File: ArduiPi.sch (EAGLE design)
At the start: 59 parts, among them IC1 DS2482-100S, IC2 AVR-MEGA8-PPTH, J1 VIN, J3 ISP, Q1 BS170, Q2 BS170, Q3 BS170, Q4 BS170, U1 LD1117 3V3, U2 78M05, U3 TXB0108, U4 TXB0108, Y1 16MHz

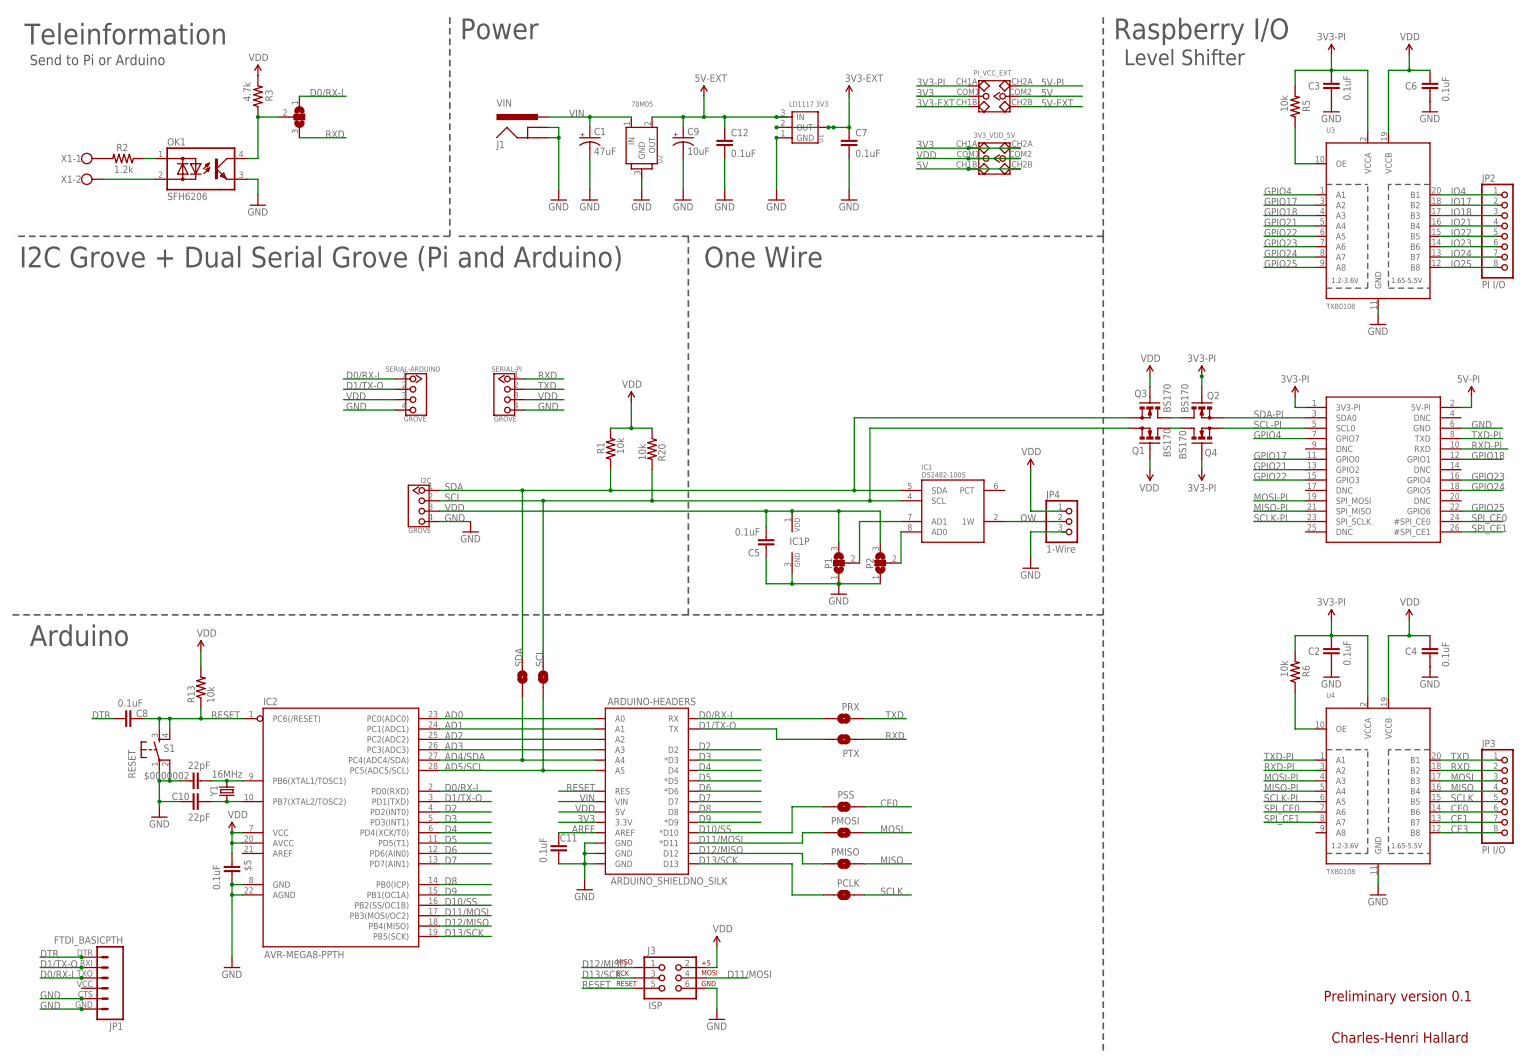
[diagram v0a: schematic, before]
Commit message: Final Design
Final Design
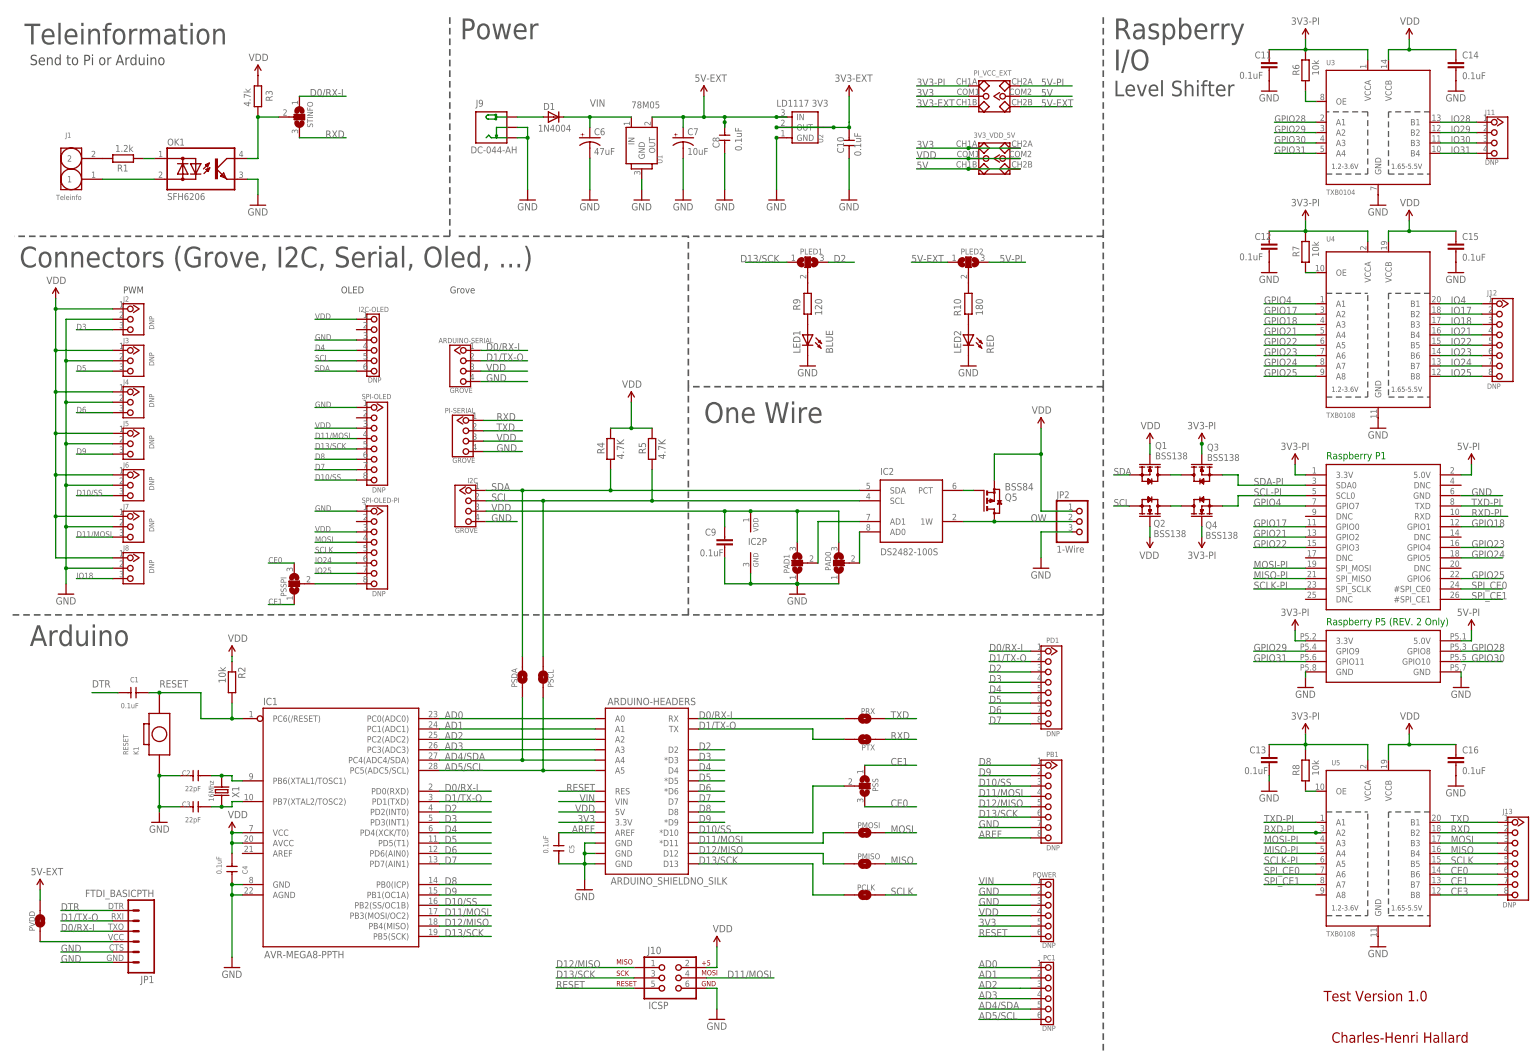
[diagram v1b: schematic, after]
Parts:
- removed $0000002: 22pF, SparkFun:CAPPTH2
- removed $5: 0.1uF, SparkFun:CAPPTH2
- removed JP3: PI I/O, adafruit:PINHD-1X8BIG
- removed JP4: 1-Wire, adafruit:PINHD-1X3
- removed P1, P2: (no value), Seeedstudio-Discreter.rpt:PAD-SOLDERJUMPER-2WAYT
- removed R13, R20: 10k, SparkFun:RESISTORAXIAL-0.3
- removed RASPBERRY: RASPBERRYPI_BB, microbuilder:RASPBERRYPI_BB
- removed S1: RESET, SparkFun:TAC_SWITCHPTH
- removed SERIAL-ARDUINO, SERIAL-PI: GROVE, Connector:TWIG-2.0-LEADED
- removed Y1: 16MHz, SparkFun:CRYSTALHC49US
- added ARDUINO-SERIAL, PI-SERIAL: GROVE, Connector:TWIG-2.0-LEADED
- added C13, C14, C15, C16: 0.1uF, resistor:C-EUC0603
- added D1: 1N4004, adafruit:1N4004
- added I2C-OLED, PC1, POWER: DNP, Seeedstudio-Connector:HEADER-6P-2.54
- added J10: ICSP, SparkFun:AVR_SPI_PRG_6PTH
- added J11: DNP, Seeedstudio-Connector:HEADER-4P-80/40MIL
- added J12, J13, PB1, PD1, SPI-OLED, SPI-OLED-PI: DNP, Seeedstudio-Connector:HEADER-8P-2.54
- added J2, J4, J5, J6, J7, J8: DNP, Seeedstudio-Connector:HEADER-3P-2.54
- added J9: DC-044-AH, For_Test_Albert:DC-044
- added K1: RESET, Seeedstudio-Discrete.rpt:BOTTON-2P-90
- added LED1: BLUE, led:LEDCHIP-LED0603
- added LED2: RED, led:LEDCHIP-LED0603
- added PAD1: PAD1, Seeedstudio-Discreter.rpt:PAD-SOLDERJUMPER-2WAYS
- added PAD2: PAD0, Seeedstudio-Discreter.rpt:PAD-SOLDERJUMPER-2WAYS
- added PI-P1: PI-P1, pi:RASPBERRYPI_BV2
- added PLED1: PLED1, Seeedstudio-Discreter.rpt:PAD-SOLDERJUMPER-2WAYS
- added PLED2: PLED2, Seeedstudio-Discreter.rpt:PAD-SOLDERJUMPER-2WAYS
- added PSSPI: PSSPI, Seeedstudio-Discreter.rpt:PAD-SOLDERJUMPER-2WAYS
- added PVDD: PVDD, Seeedstudio-Discreter.rpt:PAD-SOLDERJUMPERNC
- added Q5: BSS84, transistor-small-signal:BSS84
- added R10: 180, resistor:R-EU_R0805
- added R4: 4.7K, resistor:R-EU_R0805
- added R7, R8: 10k, resistor:R-EU_R0603
- added R9: 120, resistor:R-EU_R0805
- added U5: TXB0108, adafruit:TXB0108PWR
- C1: value 47uF -> 0.1uF; device SparkFun:CAP_POLPTH1 -> Seeedstudio-Discrete.rpt:C'1.4'
- C10: value 22pF -> 0.1uF; device SparkFun:CAPPTH2 -> Seeedstudio-Discrete.rpt:C'1.4'
- C11, C12: device SparkFun:CAPPTH2 -> resistor:C-EUC0603
- C2, C3: value 0.1uF -> 22pF; device SparkFun:CAPPTH2 -> Seeedstudio-Discrete.rpt:C'1.4'
- C4, C5, C8: device SparkFun:CAPPTH2 -> Seeedstudio-Discrete.rpt:C'1.4'
- C6: value 0.1uF -> 47uF; device SparkFun:CAPPTH2 -> SparkFun:CAP_POLPTH2
- C7: value 0.1uF -> 10uF; device SparkFun:CAPPTH2 -> SparkFun:CAP_POLPTH2
- C9: value 10uF -> 0.1uF; device SparkFun:CAP_POLPTH1 -> resistor:C-EUC0603
- IC1: value DS2482-100S -> AVR-MEGA8-PPTH; device 1wire:DS2482-100S -> SparkFun:AVR-MEGA8-PPTH
- IC2: value AVR-MEGA8-PPTH -> DS2482-100S; device SparkFun:AVR-MEGA8-PPTH -> 1wire:DS2482-100S
- J1: value VIN -> Teleinfo; device SparkFun:POWER_JACKPTH_LOCK -> Seeedstudio-Connector:HEADER-2P-2.54
- J3: value ISP -> DNP; device SparkFun:AVR_SPI_PRG_6PTH -> Seeedstudio-Connector:HEADER-3P-2.54
- JP2: value PI I/O -> 1-Wire; device adafruit:PINHD-1X8BIG -> adafruit:PINHD-1X3
- PCLK: value (none) -> PCLK
- PMISO: value (none) -> PMISO
- PMOSI: value (none) -> PMOSI
- PRX: value (none) -> PRX
- PSCL: value (none) -> PSCL
- PSDA: value (none) -> PSDA
- PSS: value (none) -> PSS; device Seeedstudio-Discreter.rpt:PAD-SOLDERJUMPERNC -> Seeedstudio-Discreter.rpt:PAD-SOLDERJUMPER-2WAYS
- PTX: value (none) -> PTX
- Q1, Q2, Q3, Q4: value BS170 -> BSS138; device transistor-small-signal:BS170 -> Seeedstudio-Discreter.rpt:MOSFET-N-SOT23
- R1: value 10k -> 1.2k; device SparkFun:RESISTORAXIAL-0.3 -> resistor:R-EU_R0805
- R2: value 1.2k -> 10k; device SparkFun:RESISTORAXIAL-0.3 -> resistor:R-EU_R0805
- R3: device SparkFun:RESISTORAXIAL-0.3 -> resistor:R-EU_R0805
- R5: value 10k -> 4.7K; device SparkFun:RESISTORAXIAL-0.3 -> resistor:R-EU_R0805
- R6: device SparkFun:RESISTORAXIAL-0.3 -> resistor:R-EU_R0603
- STINFO: value (none) -> STINFO; device Seeedstudio-Discreter.rpt:PAD-SOLDERJUMPER-2WAYT -> Seeedstudio-Discreter.rpt:PAD-SOLDERJUMPER-2WAYS
- U1: value LD1117 3V3 -> 78M05; device Seeedstudio-IC:LD1117SOT223 -> SeedStudio-IC:78M05-TO252
- U2: value 78M05 -> LD1117 3V3; device SeedStudio-IC:78M05-TO252 -> Seeedstudio-IC:LD1117SOT223
- U3: value TXB0108 -> TXB0104; device adafruit:TXB0108PWR -> adafruit:TXB0104PWR
- X1: value (none) -> 16Mhz; device _c2h:CON-CLAMP-2 -> Seeedstudio-Discrete.rpt:CRYSTAL-HC49S
- renumbered SCL to PSCL, SDA to PSDA
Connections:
- new net GPIO28: PI-P1.GPIO8, U3.A1
- new net GPIO29: PI-P1.GPIO9, U3.A2
- new net GPIO30: PI-P1.GPIO10, U3.A3
- new net GPIO31: PI-P1.GPIO11, U3.A4
- new net IO28: J11.P$1, U3.B1
- new net IO29: J11.P$2, U3.B2
- new net IO30: J11.P$3, U3.B3
- new net IO31: J11.P$4, U3.B4
- new net N$14: J1.2, R1.2
- new net N$15: IC2G$1.PCT, Q5.G
- new net N$16: PLED1.2, R9.1
- new net N$17: LED1.A, R9.2
- new net N$18: LED2.A, R10.2
- new net N$19: R6.1, U3.OE
- new net N$20: PLED2.2, R10.1
- new net SSPI: PSSPI.2, SPI-OLED-PI.8
- net 3V3: now also POWER.5
- net 3V3-EXT: now also C10.2, U2.OUT, U2.TAB; no longer C7.1, U1.TAB
- net 3V3-PI: now also C11.1, C12.1, C13.1, PI-P1.3.3V@1, PI-P1.3.3V@2, Q3.G, R7.2, R8.2, U5.VCCA; no longer C2.1, C3.1, Q2.G, R5.2, RASPBERRY.3V3-PI
- net 5V-EXT: now also C7.+, C8.2, PLED2.1, PVDD.2, U1.OUT, U2.IN; no longer C12.1, C9.+, U1.IN, U2.OUT
- net 5V-PI: now also PI-P1.5.0V@1, PI-P1.5.0V@2, PLED2.3; no longer RASPBERRY.5V-PI
- net AD0: now also IC1.PC0(ADC0), PC1.1; no longer IC2.PC0(ADC0)
- net AD1: now also IC1.PC1(ADC1), PC1.2; no longer IC2.PC1(ADC1)
- net AD2: now also IC1.PC2(ADC2), PC1.3; no longer IC2.PC2(ADC2)
- net AD3: now also IC1.PC3(ADC3), PC1.4; no longer IC2.PC3(ADC3)
- net AD4/SDA: now also IC1.PC4(ADC4/SDA), PC1.5; no longer IC2.PC4(ADC4/SDA)
- net AD5/SCL: now also IC1.PC5(ADC5/SCL), PC1.6; no longer IC2.PC5(ADC5/SCL)
- net AREF: now also C5.2, PB1.8; no longer C11.1
- net CE0: now also J13.6, PSS.3, PSSPI.3, U5.B6; no longer JP3.6, PSS.1, U4.B6
- net CE1: now also J13.7, PSS.1, PSSPI.1, U5.B7; no longer JP3.7, U4.B7
- net CE3: now also J13.8, U5.B8; no longer JP3.8, U4.B8
- net D0/RX-I: now also ARDUINO-SERIAL.1, IC1.PD0(RXD), PD1.1; no longer IC2.PD0(RXD)
- net D1/TX-O: now also ARDUINO-SERIAL.2, IC1.PD1(TXD), PD1.2; no longer IC2.PD1(TXD)
- net D10/SS: now also IC1.PB2(SS/OC1B), J6.P$3, PB1.3, SPI-OLED.8; no longer IC2.PB2(SS/OC1B)
- net D11/MOSI: now also IC1.PB3(MOSI/OC2), J10.4, J7.P$3, PB1.4, SPI-OLED.4; no longer IC2.PB3(MOSI/OC2), J3.4
- net D12/MISO: now also IC1.PB4(MISO), J10.1, PB1.5; no longer IC2.PB4(MISO), J3.1
- net D13/SCK: now also IC1.PB5(SCK), J10.3, PB1.6, PLED1.1, SPI-OLED.5; no longer IC2.PB5(SCK), J3.3
- net D2: now also IC1.PD2(INT0), PD1.3, PLED1.3; no longer IC2.PD2(INT0)
- net D3: now also IC1.PD3(INT1), J2.P$3, PD1.4; no longer IC2.PD3(INT1)
- net D4: now also I2C-OLED.4, IC1.PD4(XCK/T0), PD1.5; no longer IC2.PD4(XCK/T0)
- net D5: now also IC1.PD5(T1), J3.P$3, PD1.6; no longer IC2.PD5(T1)
- net D6: now also IC1.PD6(AIN0), J4.P$3, PD1.7; no longer IC2.PD6(AIN0)
- net D7: now also IC1.PD7(AIN1), PD1.8, SPI-OLED.7; no longer IC2.PD7(AIN1)
- net D8: now also IC1.PB0(ICP), PB1.1, SPI-OLED.6; no longer IC2.PB0(ICP)
- net D9: now also IC1.PB1(OC1A), J5.P$3, PB1.2; no longer IC2.PB1(OC1A)
- net DTR: now also C1.2; no longer C8.1
- net GND: now also ARDUINO-SERIAL.4, C13.2, C14.2, C15.2, C16.2, C6.-, C7.-, C8.1, C9.2, I2C-OLED.3, IC1.AGND, IC1.GND@1, IC2P.GND, J10.6, J2.P$2, J3.P$2, J4.P$2, J5.P$2, J6.P$2, J7.P$2, J8.P$2, J9.-, J9.CDN, JP2.3, K1.1, LED1.C, LED2.C, PAD1.1, PAD2.1, PB1.7, PI-P1.GND, PI-P1.GND@2, PI-P1.GND@3, PI-SERIAL.4, POWER.2, POWER.3, SPI-OLED-PI.1, SPI-OLED.1, U5.GND; no longer $0000002.1, $5.1, C1.-, C6.1, C7.2, C9.-, IC1P.GND, IC2.AGND, IC2.GND@1, J1.GND, J1.GNDBREAK, J3.6, P1.1, P2.1, RASPBERRY.GND, S1.1, S1.2, SERIAL-ARDUINO.4, SERIAL-PI.4
- net GPIO17: now also PI-P1.GPIO0, U4.A2; no longer RASPBERRY.GPIO0, U3.A2
- net GPIO18: now also PI-P1.GPIO1, U4.A3; no longer RASPBERRY.GPIO1, U3.A3
- net GPIO21: now also PI-P1.GPIO2, U4.A4; no longer RASPBERRY.GPIO2, U3.A4
- net GPIO22: now also PI-P1.GPIO3, U4.A5; no longer RASPBERRY.GPIO3, U3.A5
- net GPIO23: now also PI-P1.GPIO4, U4.A6; no longer RASPBERRY.GPIO4, U3.A6
- net GPIO24: now also PI-P1.GPIO5, U4.A7; no longer RASPBERRY.GPIO5, U3.A7
- net GPIO25: now also PI-P1.GPIO6, U4.A8; no longer RASPBERRY.GPIO6, U3.A8
- net GPIO4: now also PI-P1.GPIO7, U4.A1; no longer RASPBERRY.GPIO7, U3.A1
- net IO17: now also J12.2, U4.B2; no longer JP2.2, U3.B2
- net IO18: now also J12.3, J8.P$3, U4.B3; no longer JP2.3, U3.B3
- net IO21: now also J12.4, U4.B4; no longer JP2.4, U3.B4
- net IO22: now also J12.5, U4.B5; no longer JP2.5, U3.B5
- net IO23: now also J12.6, U4.B6; no longer JP2.6, U3.B6
- net IO24: now also J12.7, SPI-OLED-PI.6, U4.B7; no longer JP2.7, U3.B7
- net IO25: now also J12.8, SPI-OLED-PI.7, U4.B8; no longer JP2.8, U3.B8
- net IO4: now also J12.1, U4.B1; no longer JP2.1, U3.B1
- net MISO: now also J13.4, U5.B4; no longer JP3.4, U4.B4
- net MISO-PI: now also PI-P1.SPI_MISO, U5.A4; no longer RASPBERRY.SPI_MISO
- net MOSI: now also J13.3, SPI-OLED-PI.4, U5.B3; no longer JP3.3, U4.B3
- net MOSI-PI: now also PI-P1.SPI_MOSI, U5.A3; no longer RASPBERRY.SPI_MOSI
- net N$10: now also JP1.4, PVDD.1; no longer R2.2, X1-1.KL
- net N$11: now also IC2G$1.AD1, PAD1.2; no longer IC1G$1.AD1, P1.2
- net N$12: now also D1.A, J9.+; no longer U1.OUT
- net N$13: now also R8.1, U5.OE; no longer R6.1, U4.OE
- net N$2: now also IC2G$1.AD0, PAD2.2; no longer IC1G$1.AD0, P2.2
- net N$3: now also C3.1, IC1.PB7(XTAL2/TOSC2), X1.1; no longer $0000002.2, IC2.PB6(XTAL1/TOSC1), Y1.2
- net N$4: now also C2.1, IC1.PB6(XTAL1/TOSC1), X1.2; no longer C10.2, IC2.PB7(XTAL2/TOSC2), Y1.1
- net N$5: now also Q1.D; no longer Q2.D
- net N$6: now also Q2.D; no longer Q1.D
- net N$7: now also R7.1, U4.OE; no longer R5.1, U3.OE
- net N$8: now also R1.1; no longer R2.1
- net N$9: now also J1.1; no longer X1-2.KL
- net OW: now also IC2G$1.1W, JP2.2, Q5.D; no longer IC1G$1.1W, JP4.2
- net RESET: now also C1.1, IC1.PC6(/RESET), J10.5, K1.2, POWER.6, R2.2; no longer C8.2, IC2.PC6(/RESET), J3.5, R13.1, S1.3, S1.4
- net RXD: now also J13.2, PI-SERIAL.1, U5.B2; no longer JP3.2, U4.B2
- net RXD-PI: now also PI-P1.RXD, U5.A2; no longer RASPBERRY.RXD
- net SCL: now also I2C-OLED.5, IC2G$1.SCL, Q2.S, R5.1; no longer IC1G$1.SCL, Q1.S, R20.2
- net SCL-PI: now also PI-P1.SCL0; no longer RASPBERRY.SCL0
- net SCLK: now also J13.5, SPI-OLED-PI.5, U5.B5; no longer JP3.5, U4.B5
- net SCLK-PI: now also PI-P1.SPI_SCLK, U5.A5; no longer RASPBERRY.SPI_SCLK
- net SDA: now also I2C-OLED.6, IC2G$1.SDA, Q1.S, R4.1; no longer IC1G$1.SDA, Q3.S, R1.1
- net SDA-PI: now also PI-P1.SDA0, Q3.S; no longer Q2.S, RASPBERRY.SDA0
- net SPI_CE0: now also PI-P1.#SPI_CE0, U5.A6; no longer RASPBERRY.#SPI_CE0
- net SPI_CE1: now also PI-P1.#SPI_CE1, U5.A7; no longer RASPBERRY.#SPI_CE1
- net TXD: now also J13.1, PI-SERIAL.2, U5.B1; no longer JP3.1, U4.B1
- net TXD-PI: now also PI-P1.TXD, U5.A1; no longer RASPBERRY.TXD
- net VDD: now also ARDUINO-SERIAL.3, C14.1, C15.1, C16.1, C9.1, I2C-OLED.1, IC1.AVCC, IC1.VCC@1, IC2P.VDD, J10.2, J2.P$1, J3.P$1, J4.P$1, J5.P$1, J6.P$1, J7.P$1, J8.P$1, JP2.1, PAD1.3, PAD2.3, PI-SERIAL.3, POWER.4, Q2.G, Q5.S, R2.1, R4.2, R5.2, SPI-OLED-PI.3, SPI-OLED.3, U5.VCCB; no longer $5.2, C5.2, C6.2, IC1P.VDD, IC2.AVCC, IC2.VCC@1, J3.2, JP4.1, P1.3, P2.3, Q3.G, R1.2, R13.2, R20.1, SERIAL-ARDUINO.3, SERIAL-PI.3
- net VIN: now also C6.+, D1.C, POWER.1, U1.IN; no longer C1.+, J1.PWR, U2.IN
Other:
- note added: "Connectors (Grove, I2C, Serial, Oled, ...)"
- note added: "Grove"
- note added: "OLED"
- note added: "PWM"
- note added: "Raspberry P1"
- note added: "Raspberry P5 (REV. 2 Only)"
- note added: "Test Version 1.0"
- note removed: "I2C Grove + Dual Serial Grove (Pi and Arduino)"
- note removed: "Preliminary version 0.1"
- moved on the sheet: C11, C12, I2C, JP1, PCLK, PMISO, PMOSI, PRX, PTX, U4
